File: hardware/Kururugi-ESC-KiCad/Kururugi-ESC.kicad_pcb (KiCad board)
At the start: 6 copper layers, 37.9 x 23.6 mm, 141 parts, among them J1 Conn_01x01, J10 Conn_01x01, J11 Conn_01x01, J2 Conn_01x01, J3 Conn_01x01, J4 Conn_01x01, J5 Conn_01x01, J6 Conn_01x01, J7 Conn_01x01, J8 JTAG_TC2030, J9 Conn_01x01, Q1 CSD18540Q5B, Q2 CSD18540Q5B, Q3 CSD18540Q5B, Q4 CSD18540Q5B, Q5 CSD18540Q5B, Q6 CSD18540Q5B, U1 STM32G474CEU6, U2 LM5160A, U3 TPS7B92033, U4 2EDL8024, U5 2EDL8024, U6 2EDL8024, X1 16MHz

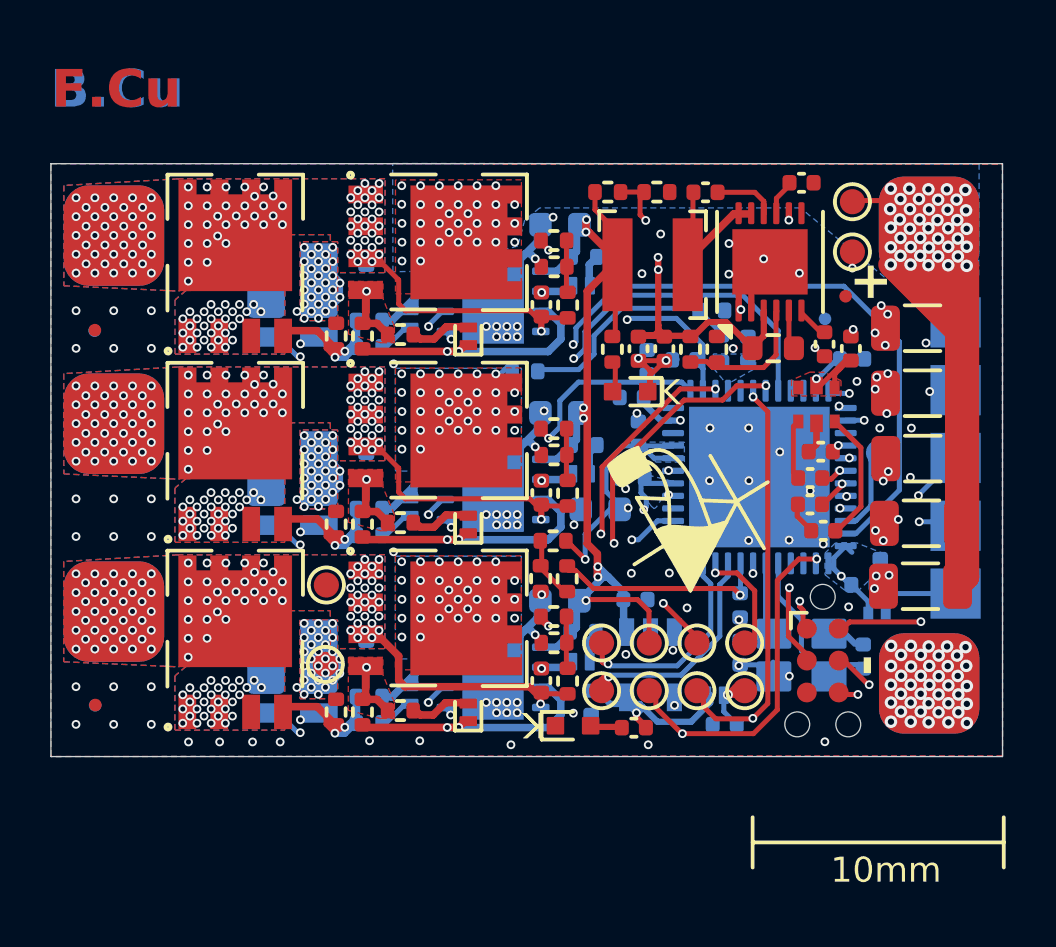
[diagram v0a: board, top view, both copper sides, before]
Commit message: PCB Improvments
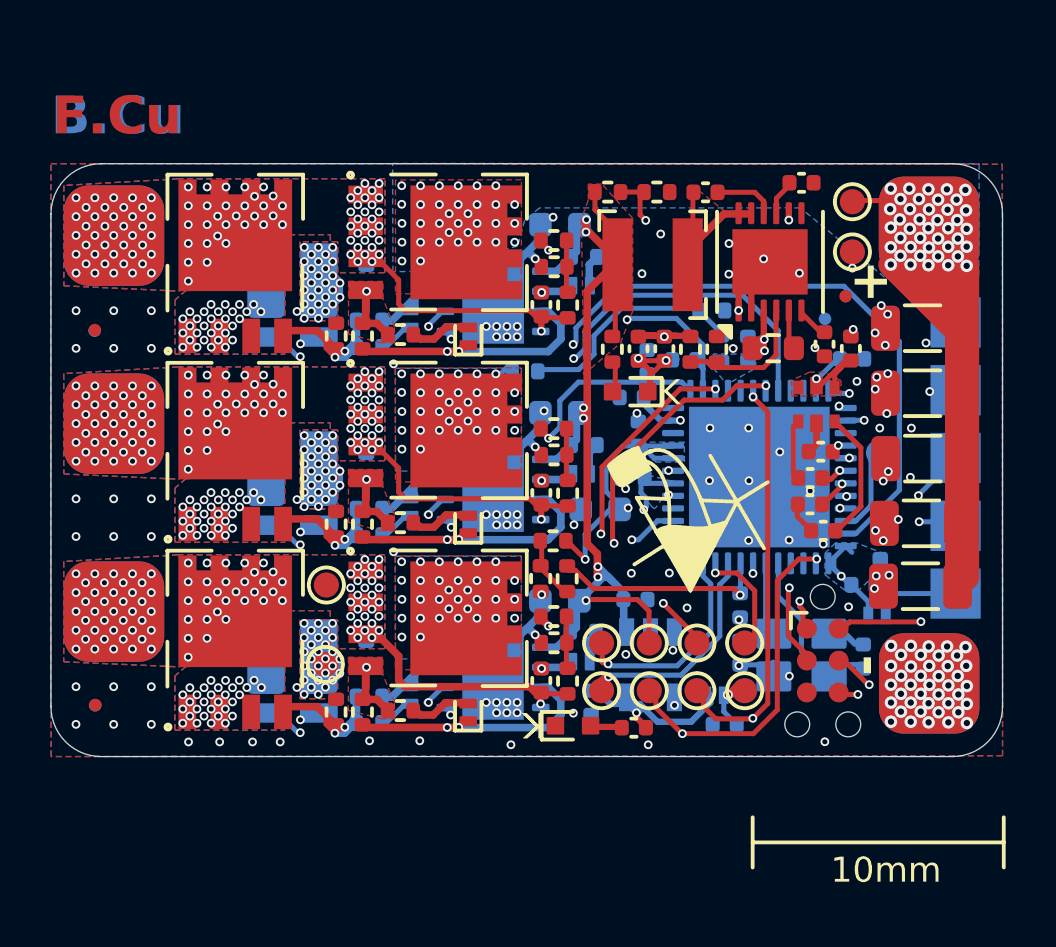
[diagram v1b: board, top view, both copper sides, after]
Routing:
- net VBAT: track 56.9 -> 51.5 mm, vias 142 -> 143
- added copper zone on F.Cu, net /SW
- added copper zone on F.Cu, net VBUCK
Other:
- outline, holes or cut-outs redrawn
- board text removed: "Edge.Cuts"
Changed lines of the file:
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@@
 		(layer "F.SilkS")
 	)
-	(gr_rect
-		(start 47.948628 24.289474)
-		(end 85.848628 47.902474)
+	(gr_line
+		(start 49.948628 24.289474)
+		(end 83.848628 24.289474)
+		(stroke
+			(width 0.05)
+			(type default)
+		)
+		(layer "Edge.Cuts")
+	)
+	(gr_arc
+		(start 47.948628 26.289474)
+		(mid 48.534425 24.875287)
+		(end 49.948628 24.289474)
+		(stroke
+			(width 0.05)
+			(type default)
+		)
+		(layer "Edge.Cuts")
+	)
+	(gr_arc
+		(start 83.848628 24.289474)
+		(mid 85.262842 24.87526)
+		(end 85.848628 26.289474)
+		(stroke
+			(width 0.05)
+			(type default)
+		)
+		(layer "Edge.Cuts")
+	)
+	(gr_arc
+		(start 85.848628 45.902474)
+		(mid 85.262852 47.316714)
+		(end 83.848628 47.902474)
+		(stroke
+			(width 0.05)
+			(type default)
+		)
+		(layer "Edge.Cuts")
+	)
+	(gr_line
+		(start 85.848628 26.289474)
+		(end 85.848628 45.902474)
+		(stroke
+			(width 0.05)
+			(type default)
+		)
+		(layer "Edge.Cuts")
+	)
+	(gr_arc
+		(start 49.948628 47.902474)
+		(mid 48.534414 47.316688)
+		(end 47.948628 45.902474)
+		(stroke
+			(width 0.05)
+			(type default)
+		)
+		(layer "Edge.Cuts")
+	)
+	(gr_line
+		(start 83.848628 47.902474)
+		(end 49.948628 47.902474)
+		(stroke
+			(width 0.05)
+			(type default)
+		)
+		(layer "Edge.Cuts")
+	)
+	(gr_line
+		(start 47.948628 45.902474)
+		(end 47.948628 26.289474)
 		(stroke
 			(width 0.05)
 			(type default)
 		)
-		(fill no)
 		(layer "Edge.Cuts")
 	)
 	(gr_text "F.Cu"
-		(at 47.97 22.2 0)
+		(at 48 23.26 0)
 		(layer "F.Cu")
 		(effects
@@
 	)
 	(gr_text "B.Cu"
-		(at 47.92 22.2 0)
+		(at 47.95 23.26 0)
 		(layer "B.Cu")
 		(effects
@@
 	)
 	(gr_text "In1.Cu"
-		(at 47.92 22.2 0)
+		(at 47.95 23.26 0)
 		(layer "In1.Cu")
 		(effects
@@
 	)
 	(gr_text "In2.Cu"
-		(at 47.92 22.2 0)
+		(at 47.95 23.26 0)
 		(layer "In2.Cu")
 		(effects
@@
 	)
 	(gr_text "-"
-		(at 81.588628 45.499474 90)
+		(at 81.42 45.55 90)
 		(layer "B.SilkS")
 		(effects
@@
 	)
 	(gr_text "In3.Cu"
-		(at 47.92 22.2 0)
+		(at 47.95 23.26 0)
 		(layer "In3.Cu")
 		(effects
@@
 	)
 	(gr_text "In4.Cu"
-		(at 47.92 22.2 0)
+		(at 47.95 23.26 0)
 		(layer "In4.Cu")
 		(effects
@@
 		)
 	)
-	(gr_text "Edge.Cuts"
-		(at 47.92 22.2 0)
-		(layer "Edge.Cuts")
-		(effects
-			(font
-				(size 1.5 1.5)
-				(thickness 0.3)
-				(bold yes)
-			)
-			(justify left bottom)
-		)
-	)
 	(segment
 		(start 69.258628 26.539474)
@@
 	)
 	(via
-		(at 75.428628 30.099474)
+		(at 75.337628 30.136974)
 		(size 0.35)
 		(drill 0.2)
@@
 	)
 	(segment
-		(start 72.136628 30.719474)
-		(end 72.136628 30.971474)
-		(width 0.25)
-		(layer "F.Cu")
-		(net 9)
-	)
-	(segment
 		(start 84.420828 28.357837)
 		(end 84.420828 40.752274)
@@
 	)
 	(segment
-		(start 73.564878 31.142224)
-		(end 74.107628 30.599474)
-		(width 0.25)
-		(layer "F.Cu")
-		(net 9)
-	)
-	(segment
 		(start 84.136628 30.497474)
 		(end 82.118628 28.479474)
@@
 	)
 	(segment
+		(start 76.37 31.74)
+		(end 76.18 31.93)
+		(width 0.2)
+		(layer "F.Cu")
+		(net 9)
+	)
+	(segment
 		(start 71.459378 31.142224)
 		(end 73.564878 31.142224)
@@
 	)
 	(segment
-		(start 72.136628 28.025474)
-		(end 72.136628 30.719474)
-		(width 0.25)
-		(layer "F.Cu")
-		(net 9)
-	)
-	(segment
 		(start 84.136628 30.840437)
 		(end 84.136628 28.642037)
@@
 	)
 	(segment
-		(start 74.847628 30.599474)
-		(end 75.887628 31.639474)
-		(width 0.25)
-		(layer "F.Cu")
-		(net 9)
-	)
-	(segment
 		(start 75.887628 31.639474)
 		(end 75.988628 31.639474)
@@
 	)
 	(segment
-		(start 74.107628 30.599474)
-		(end 74.847628 30.599474)
-		(width 0.25)
-		(layer "F.Cu")
-		(net 9)
-	)
-	(segment
-		(start 72.136628 30.971474)
-		(end 71.978628 31.129474)
-		(width 0.25)
-		(layer "F.Cu")
-		(net 9)
-	)
-	(segment
-		(start 72.129628 28.018474)
-		(end 72.136628 28.025474)
-		(width 0.25)
+		(start 76.18 31.93)
+		(end 76.17 31.93)
+		(width 0.2)
 		(layer "F.Cu")
 		(net 9)
@@
 	)
 	(segment
-		(start 72.136628 30.895474)
-		(end 72.407378 31.166224)
+		(start 72.86 31.142224)
+		(end 72.559378 31.142224)
 		(width 0.25)
 		(layer "F.Cu")
@@
 	)
 	(segment
+		(start 76.36 31.29)
+		(end 76.36 31.56)
+		(width 0.2)
+		(layer "F.Cu")
+		(net 9)
+	)
+	(segment
 		(start 84.420828 40.752274)
 		(end 84.056628 41.116474)
@@
 	)
 	(segment
+		(start 76.36 31.56)
+		(end 76.280526 31.639474)
+		(width 0.2)
+		(layer "F.Cu")
+		(net 9)
+	)
+	(segment
 		(start 71.459378 31.142224)
 		(end 71.425378 31.176224)
@@
 	)
 	(segment
-		(start 71.472128 31.129474)
-		(end 71.425378 31.176224)
-		(width 0.25)
+		(start 76.280526 31.639474)
+		(end 75.888628 31.639474)
+		(width 0.2)
 		(layer "F.Cu")
 		(net 9)
 	)
 	(segment
-		(start 72.136628 30.719474)
-		(end 72.136628 30.895474)
+		(start 71.472128 31.129474)
+		(end 71.425378 31.176224)
 		(width 0.25)
 		(layer "F.Cu")
@@
 	)
 	(via
+		(at 76.37 31.74)
+		(size 0.35)
+		(drill 0.2)
+		(layers "F.Cu" "B.Cu")
+		(net 9)
+	)
+	(via
 		(at 62.668413 35.659744)
 		(size 0.35)
@@
 	)
 	(via
-		(at 72.129628 28.018474)
-		(size 0.35)
-		(drill 0.2)
-		(layers "F.Cu" "B.Cu")
-		(net 9)
-	)
-	(via
 		(at 61.926703 43.141696)
 		(size 0.35)
@@
 	)
 	(via
+		(at 76.36 31.29)
+		(size 0.35)
+		(drill 0.2)
+		(layers "F.Cu" "B.Cu")
+		(net 9)
+	)
+	(via
 		(at 84.044628 26.534874)
 		(size 0.5)
@@
 	)
 	(via
-		(at 72.138628 28.509474)
+		(at 72.378628 31.179474)
 		(size 0.35)
 		(drill 0.2)
@@
 	)
 	(segment
-		(start 75.140628 26.291974)
-		(end 75.712628 26.291974)
+		(start 73.311628 28.120974)
+		(end 73.311628 28.312974)
+		(width 0.5)
+		(layer "F.Cu")
+		(net 16)
+	)
+	(segment
+		(start 73.311628 27.738372)
+		(end 73.311628 28.120974)
 		(width 0.3)
 		(layer "F.Cu")
@@
 	)
 	(segment
-		(start 73.311628 28.120974)
-		(end 73.311628 28.312974)
-		(width 0.5)
+		(start 75.712628 26.291974)
+		(end 74.758026 26.291974)
+		(width 0.3)
 		(layer "F.Cu")
 		(net 16)
@@
 	)
 	(segment
-		(start 75.140628 26.291974)
-		(end 73.311628 28.120974)
+		(start 74.758026 26.291974)
+		(end 73.311628 27.738372)
 		(width 0.3)
 		(layer "F.Cu")
@@
 	)
 	(zone
+		(net 16)
+		(net_name "/SW")
+		(layer "F.Cu")
+		(hatch edge 0.5)
+		(priority 14)
+		(connect_pads yes
+			(clearance 0)
+		)
+		(min_thickness 0.25)
+		(filled_areas_thickness no)
+		(fill yes
+			(thermal_gap 0.5)
+			(thermal_bridge_width 0.5)
+		)
+		(polygon
+			(pts
+				(xy 73.54 25.5) (xy 73.38 27.59) (xy 74.1 26.96) (xy 74.8 26.3) (xy 74.83 26.22) (xy 73.65 25.28)
+			)
+		)
+	)
+	(zone
 		(net 78)
 		(net_name "/PHASE 1/GH")
@@
 			)
 		)
+	)
+	(zone
+		(net 1)
+		(net_name "VBUCK")
+		(layer "F.Cu")
+		(hatch edge 0.5)
+		(priority 15)
+		(connect_pads yes
+			(clearance 0)
+		)
+		(min_thickness 0.25)
+		(filled_areas_thickness no)
+		(fill yes
+			(thermal_gap 0.5)
+			(thermal_bridge_width 0.5)
+		)
+		(polygon
+			(pts
+				(xy 69.35 25.74) (xy 69.08 26.48) (xy 69.08 27.02) (xy 69.16 31.44) (xy 69.16 32.69) (xy 70.63 31.44)
+				(xy 71.12 30.16) (xy 71.12 26.46) (xy 69.89 25.1) (xy 69.35 25.1)
+			)
+		)
